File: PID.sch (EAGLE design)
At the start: 26 parts, among them IC1 UA741CPE4, IC2 UA741CPE4, IC3 UA741CPE4, IC4 UA741CPE4, IC5 UA741CPE4

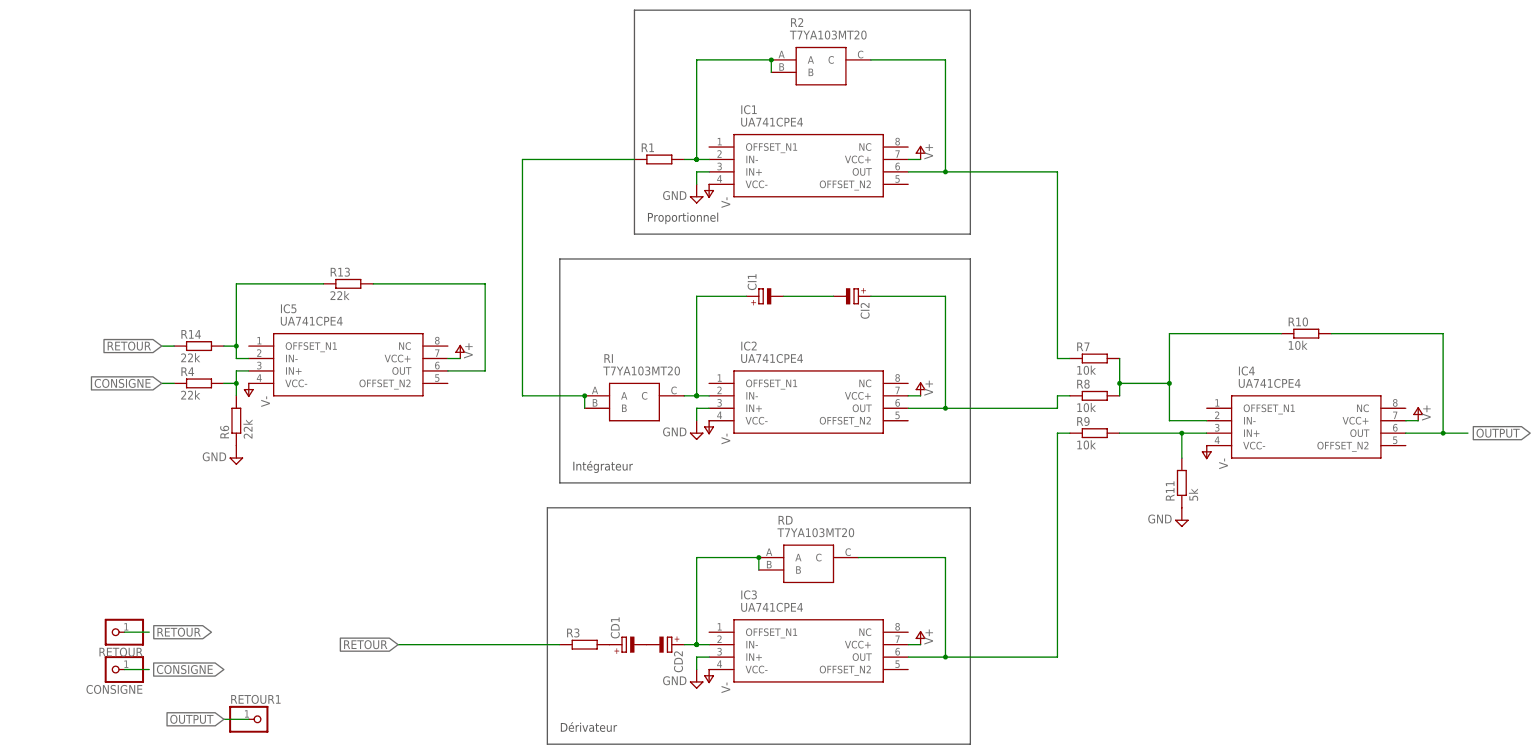
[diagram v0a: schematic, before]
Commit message: paf
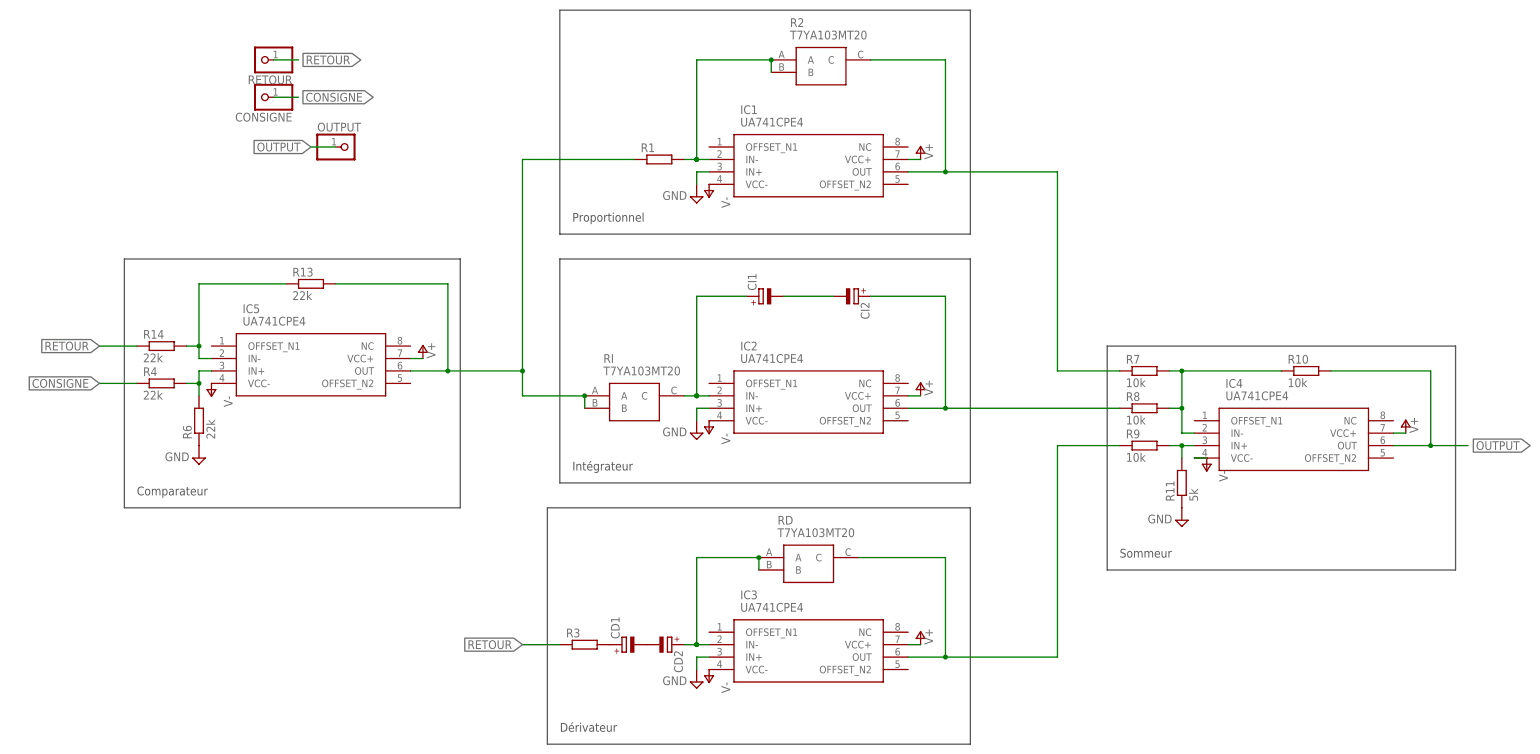
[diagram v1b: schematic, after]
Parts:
- removed RETOUR1: (no value), pinhead:PINHD-1X1
- added OUTPUT: (no value), pinhead:PINHD-1X1
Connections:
- removed net N$7 (its old number): R1.1, RI.A, RI.B
- net N$15: now also R1.1, RI.A, RI.B
- net OUTPUT: now also OUTPUT.1; no longer RETOUR1.1
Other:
- note added: "Comparateur"
- note added: "Sommeur"
- moved on the sheet: CONSIGNE, IC4, IC5, R10, R13, R14, R4, R6, R7, R8, R9, RETOUR
